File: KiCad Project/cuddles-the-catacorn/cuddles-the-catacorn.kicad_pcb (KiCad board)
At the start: 2 copper layers, 61 x 81.1 mm, 43 parts, among them U1 (Pico)

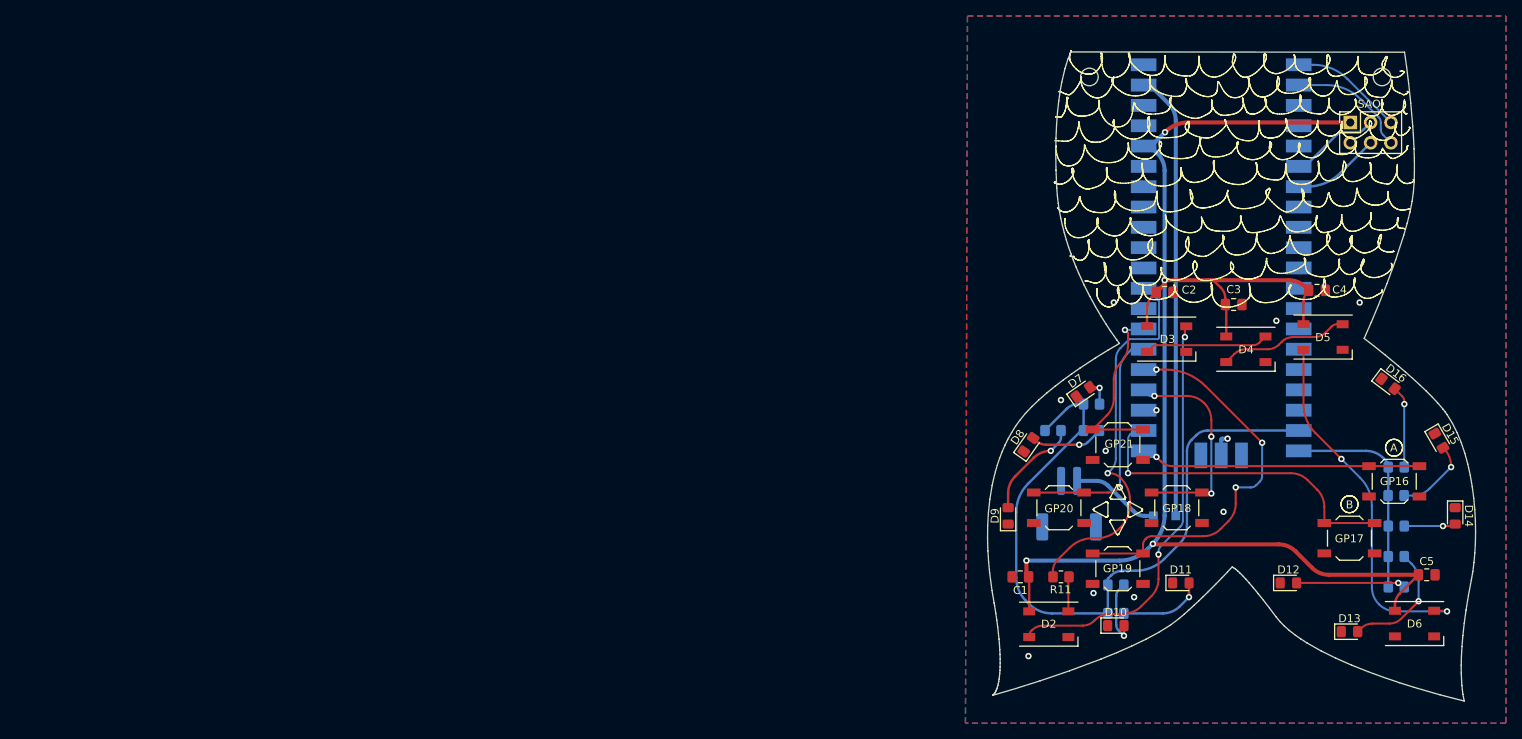
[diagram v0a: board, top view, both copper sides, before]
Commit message: First draft
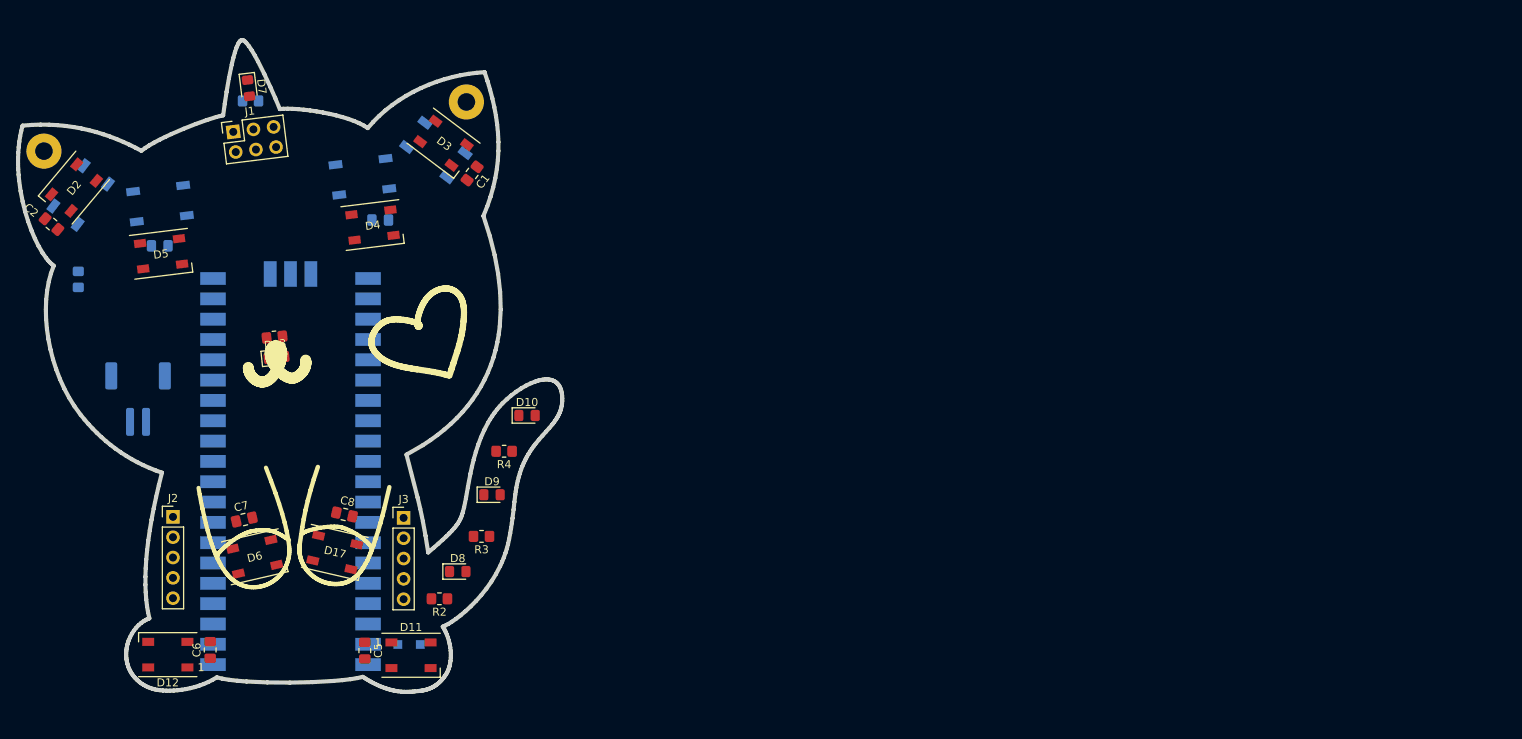
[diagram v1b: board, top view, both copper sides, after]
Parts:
- removed D14, D15, D16: LED, LED_SMD:LED_0805_2012Metric_Pad1.15x1.40mm_HandSolder
- removed Down: Down, Button_Switch_SMD:SW_SPST_TL3342
- removed R10, R6, R7, R8, R9: R, Resistor_SMD:R_0805_2012Metric_Pad1.20x1.40mm_HandSolder
- removed Right: Right, Button_Switch_SMD:SW_SPST_TL3342
- added C6: C 0.1uF, Capacitor_SMD:C_0805_2012Metric_Pad1.18x1.45mm_HandSolder, F.Cu at (93.5, 125.5)
- added C7: C 0.1uF, Capacitor_SMD:C_0805_2012Metric_Pad1.18x1.45mm_HandSolder, F.Cu at (97.8, 109.2)
- added C8: C 0.1uF, Capacitor_SMD:C_0805_2012Metric_Pad1.18x1.45mm_HandSolder, F.Cu at (110.3, 108.5)
- added D17: WS2812B, LED_SMD:LED_WS2812B_PLCC4_5.0x5.0mm_P3.2mm, F.Cu at (109.1, 113.3)
- added J2: Conn_01x05, Connector_PinHeader_2.54mm:PinHeader_1x05_P2.54mm_Vertical, F.Cu at (88.9, 108.8)
- added J3: Conn_01x05, Connector_PinHeader_2.54mm:PinHeader_1x05_P2.54mm_Vertical, F.Cu at (117.7, 109.0)
- C1, C2, C5: value C -> C 0.1uF
- C3, C4: value C -> C 0.1uF; moved to B.Cu
- D11, D12: value LED -> WS2812B; footprint LED_SMD:LED_0805_2012Metric_Pad1.15x1.40mm_HandSolder -> LED_SMD:LED_WS2812B_PLCC4_5.0x5.0mm_P3.2mm
- H1, H2: footprint MountingHole:MountingHole_2.2mm_M2 -> MountingHole:MountingHole_2.2mm_M2_Pad
- R1: value R -> R470
- R11: value R -> R470; moved to B.Cu
- R2, R3, R4, R5: value R -> R470; moved to F.Cu
- SW1: renamed from Left; value Left -> C; moved to B.Cu
- SW2: renamed from Up; value Up -> D; moved to B.Cu
- SW3: renamed from B; moved to B.Cu
- SW4: renamed from A; moved to B.Cu
- U1: value (Pico) -> SC0915
- moved SW3 164.3 mm to (77.4, 68.6), turned to 53 degrees
- moved D5 145.6 mm to (87.4, 76.0), turned to 7 degrees
- moved D6 145.2 mm to (99.1, 113.8), turned to 13 degrees
- moved D12 140.4 mm to (88.3, 126.1), turned to 180 degrees
- moved J1 139.6 mm to (96.4, 60.7), turned to 97 degrees
- moved C2 139.4 mm to (73.7, 72.2), turned to 140 degrees
- moved D13 138.4 mm to (101.8, 88.9), turned to 6 degrees
- moved C3 134.4 mm to (87.2, 75.0)
- moved D2 133.5 mm to (76.5, 67.7), turned to -130 degrees
- moved C5 133.1 mm to (112.9, 125.6), turned to -90 degrees
- moved H1 131.0 mm to (72.8, 63.1)
- moved R11 128.3 mm to (77.1, 79.1), turned to -90 degrees
- moved SW4 126.7 mm to (121.8, 63.0), turned to -37 degrees
- moved U1 119.4 mm to (103.6, 103.2), turned to 0 degrees
- moved SW1 118.6 mm to (87.3, 69.7), turned to 7 degrees
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- renumbered Battery to BT1, SAO to J1
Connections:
- BT1 pad MP: GND -> (no net)
- D11 pad 1: GND -> +3V3
- D12 pad 1: GND -> +3V3
- D12 pad 2: Net-(D12-Pad2) -> unconnected-(D12-Pad2)
- D6 pad 2: unconnected-(D6-Pad2) -> Net-(D6-Pad2)
- R2 pad 2: Net-(R1-Pad2) -> Net-(U1-Pad20)
- R3 pad 2: Net-(R1-Pad2) -> Net-(U1-Pad20)
- R4 pad 2: Net-(R1-Pad2) -> Net-(U1-Pad20)
- R5 pad 1: Net-(D11-Pad2) -> Net-(D13-Pad2)
- R5 pad 2: Net-(R1-Pad2) -> Net-(U1-Pad17)
- SW3 pad 1: Net-(SW5-Pad1) -> Net-(U1-Pad25)
- SW4 pad 1: Net-(SW6-Pad1) -> Net-(SW4-Pad1)
- U1 pad 10: unconnected-(U1-Pad10) -> Net-(U1-Pad10)
- U1 pad 11: unconnected-(U1-Pad11) -> Net-(U1-Pad11)
- U1 pad 12: unconnected-(U1-Pad12) -> Net-(U1-Pad12)
- U1 pad 14: unconnected-(U1-Pad14) -> Net-(U1-Pad14)
- U1 pad 15: unconnected-(U1-Pad15) -> Net-(U1-Pad15)
- U1 pad 17: unconnected-(U1-Pad17) -> Net-(U1-Pad17)
- U1 pad 20: Net-(R10-Pad2) -> Net-(U1-Pad20)
- U1 pad 21: Net-(SW6-Pad1) -> unconnected-(U1-Pad21)
- U1 pad 22: Net-(SW5-Pad1) -> unconnected-(U1-Pad22)
- U1 pad 24: Net-(SW3-Pad1) -> Net-(SW4-Pad1)
- U1 pad 25: Net-(SW4-Pad1) -> Net-(U1-Pad25)
- U1 pad 4: unconnected-(U1-Pad4) -> Net-(U1-Pad4)
- U1 pad 5: unconnected-(U1-Pad5) -> Net-(U1-Pad5)
- U1 pad 9: unconnected-(U1-Pad9) -> Net-(U1-Pad9)
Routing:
- net +3V3: track 179.2 -> 0.00 mm, vias 4 -> 0
- net Net-(R1-Pad2): track 87.0 -> 0.00 mm
- net Net-(D1-Pad1): track 55.8 -> 0.00 mm
- net Net-(D2-Pad2): track 52.7 -> 0.00 mm, vias 2 -> 0
- net Net-(SW4-Pad1): track 50.2 -> 0.00 mm, vias 3 -> 0
- net /LED_DATA_1: track 49.2 -> 0.00 mm, vias 1 -> 0
- net Net-(D5-Pad2): track 45.5 -> 0.00 mm, vias 2 -> 0
- net Net-(SW5-Pad1): track 43.3 -> 0.00 mm, vias 1 -> 0
- net Net-(SW6-Pad1): track 35.2 -> 0.00 mm, vias 1 -> 0
- net Net-(SW1-Pad1): track 30.2 -> 0.00 mm, vias 1 -> 0
- net Net-(R10-Pad2): track 27.4 -> 0.00 mm
- net Net-(SW3-Pad1): track 27.2 -> 0.00 mm, vias 3 -> 0
- net Net-(SW2-Pad1): track 22.7 -> 0.00 mm, vias 1 -> 0
- net Net-(D4-Pad2): track 16.1 -> 0.00 mm
- net Net-(D3-Pad2): track 15.5 -> 0.00 mm
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- removed copper zone on B.Cu, net GND
- removed copper zone on F.Cu, net GND
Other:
- board size 61 x 81.1 mm -> 68 x 81.5 mm
- board text added: "Cuddles the Catacorn by @GalaxyAllie and friends"
- board text removed: "+"
- board text removed: "GP16"
- board text removed: "GP17"
- board text removed: "GP18"
- board text removed: "GP19"
- board text removed: "GP20"
- board text removed: "GP21"
- board text removed: "Molly the Mermaid by @GalaxyAllie and friends"
